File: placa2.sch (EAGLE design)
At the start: 9 parts

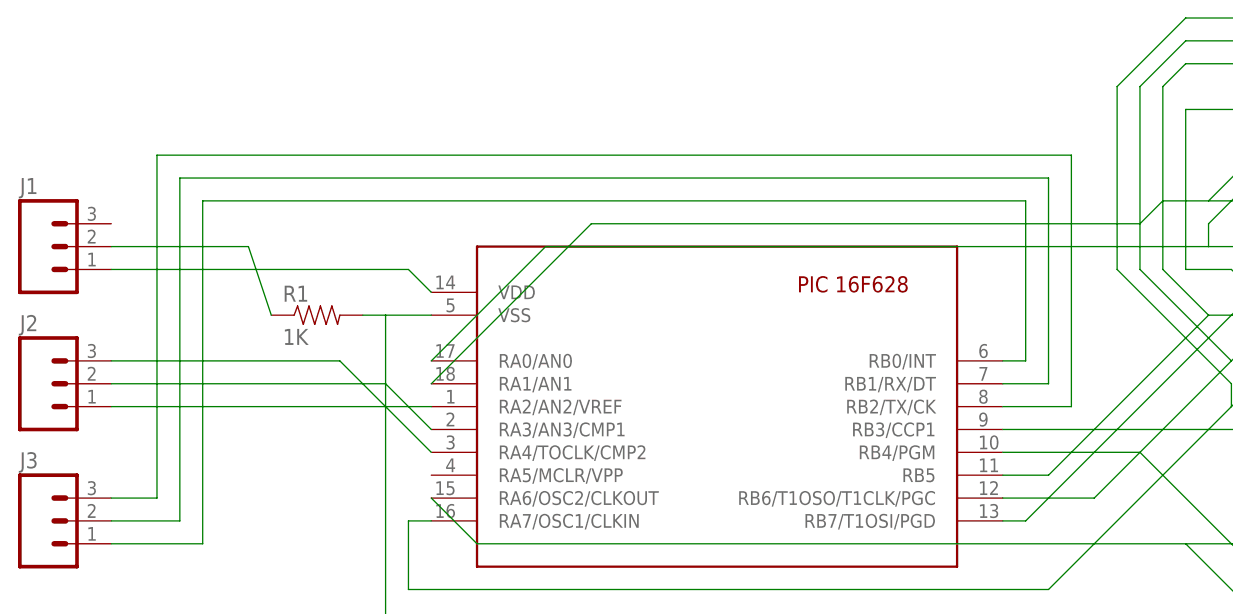
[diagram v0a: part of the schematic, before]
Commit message: feito
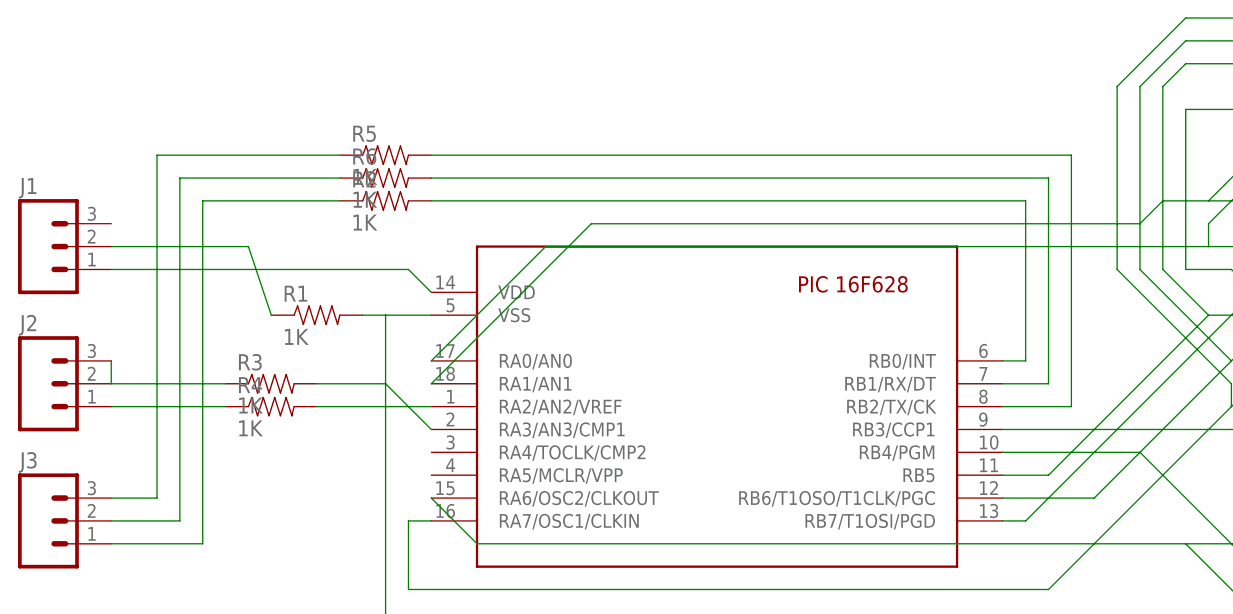
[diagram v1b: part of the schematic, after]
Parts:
- added R2, R3, R4, R5, R6: 1K, SparkFun-Resistors:1KOHM-1/4W-1%(PTH)
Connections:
- new net N$14: J3.2, R6.1
- new net N$16: J3.1, R2.1
- new net N$21: R3.2, U$1.RA3/AN3/CMP1
- new net N$24: R4.2, U$1.RA2/AN2/VREF
- net N$3: now also R4.1; no longer U$1.RA2/AN2/VREF
- net N$5: now also J2.3, R3.1; no longer J2.2, U$1.RA3/AN3/CMP1
- net N$6: now also J3.3, R5.1; no longer J2.3, U$1.RA4/TOCLK/CMP2
- net N$7: now also R2.2; no longer J3.1
- net N$8: now also R6.2; no longer J3.2
- net N$9: now also R5.2; no longer J3.3
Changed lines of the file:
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@@
 <classes>
 <class number="0" name="default" width="0.8" drill="0">
-<clearance class="0" value="0.3"/>
+<clearance class="0" value="0.4"/>
 </class>
 </classes>
@@
 <part name="T1" library="transistor" deviceset="*-PNP-" device="TO92-EBC" technology="BC558B"/>
 <part name="T2" library="transistor" deviceset="*-PNP-" device="TO92-EBC" technology="BC558B"/>
+<part name="R3" library="SparkFun-Resistors" deviceset="1KOHM-1/4W-1%(PTH)" device="" value="1K"/>
+<part name="R4" library="SparkFun-Resistors" deviceset="1KOHM-1/4W-1%(PTH)" device="" value="1K"/>
+<part name="R5" library="SparkFun-Resistors" deviceset="1KOHM-1/4W-1%(PTH)" device="" value="1K"/>
+<part name="R6" library="SparkFun-Resistors" deviceset="1KOHM-1/4W-1%(PTH)" device="" value="1K"/>
+<part name="R2" library="SparkFun-Resistors" deviceset="1KOHM-1/4W-1%(PTH)" device="" value="1K"/>
 </parts>
 <sheets>
@@
 <instance part="T1" gate="G$1" x="109.22" y="-7.62" rot="R90"/>
 <instance part="T2" gate="G$1" x="172.72" y="-20.32" rot="R90"/>
+<instance part="R3" gate="G$1" x="-35.56" y="22.86"/>
+<instance part="R4" gate="G$1" x="-35.56" y="20.32"/>
+<instance part="R5" gate="G$1" x="-22.86" y="48.26"/>
+<instance part="R6" gate="G$1" x="-22.86" y="45.72"/>
+<instance part="R2" gate="G$1" x="-22.86" y="43.18"/>
 </instances>
 <busses>
@@
 <segment>
 <pinref part="J2" gate="J$1" pin="1"/>
-<pinref part="U$1" gate="G$1" pin="RA2/AN2/VREF"/>
-<wire x1="-53.34" y1="20.32" x2="-17.78" y2="20.32" width="0.1524" layer="91"/>
-</segment>
-</net>
-<net name="N$5" class="0">
-<segment>
-<pinref part="J2" gate="J$1" pin="2"/>
-<pinref part="U$1" gate="G$1" pin="RA3/AN3/CMP1"/>
-<wire x1="-53.34" y1="22.86" x2="-22.86" y2="22.86" width="0.1524" layer="91"/>
-<wire x1="-22.86" y1="22.86" x2="-17.78" y2="17.78" width="0.1524" layer="91"/>
-</segment>
-</net>
-<net name="N$6" class="0">
-<segment>
-<pinref part="J2" gate="J$1" pin="3"/>
-<pinref part="U$1" gate="G$1" pin="RA4/TOCLK/CMP2"/>
-<wire x1="-53.34" y1="25.4" x2="-27.94" y2="25.4" width="0.1524" layer="91"/>
-<wire x1="-27.94" y1="25.4" x2="-17.78" y2="15.24" width="0.1524" layer="91"/>
+<wire x1="-53.34" y1="20.32" x2="-40.64" y2="20.32" width="0.1524" layer="91"/>
+<pinref part="R4" gate="G$1" pin="1"/>
 </segment>
 </net>
@@
 <net name="N$7" class="0">
 <segment>
-<pinref part="J3" gate="J$1" pin="1"/>
-<wire x1="-53.34" y1="5.08" x2="-43.18" y2="5.08" width="0.1524" layer="91"/>
-<wire x1="-43.18" y1="5.08" x2="-43.18" y2="43.18" width="0.1524" layer="91"/>
-<wire x1="-43.18" y1="43.18" x2="48.26" y2="43.18" width="0.1524" layer="91"/>
+<wire x1="-17.78" y1="43.18" x2="48.26" y2="43.18" width="0.1524" layer="91"/>
 <wire x1="48.26" y1="43.18" x2="48.26" y2="25.4" width="0.1524" layer="91"/>
 <pinref part="U$1" gate="G$1" pin="RB0/INT"/>
 <wire x1="48.26" y1="25.4" x2="45.72" y2="25.4" width="0.1524" layer="91"/>
+<pinref part="R2" gate="G$1" pin="2"/>
 </segment>
 </net>
 <net name="N$8" class="0">
 <segment>
-<pinref part="J3" gate="J$1" pin="2"/>
-<wire x1="-53.34" y1="7.62" x2="-45.72" y2="7.62" width="0.1524" layer="91"/>
-<wire x1="-45.72" y1="7.62" x2="-45.72" y2="45.72" width="0.1524" layer="91"/>
-<wire x1="-45.72" y1="45.72" x2="50.8" y2="45.72" width="0.1524" layer="91"/>
+<wire x1="-17.78" y1="45.72" x2="50.8" y2="45.72" width="0.1524" layer="91"/>
 <wire x1="50.8" y1="45.72" x2="50.8" y2="22.86" width="0.1524" layer="91"/>
 <pinref part="U$1" gate="G$1" pin="RB1/RX/DT"/>
 <wire x1="50.8" y1="22.86" x2="45.72" y2="22.86" width="0.1524" layer="91"/>
+<pinref part="R6" gate="G$1" pin="2"/>
 </segment>
 </net>
 <net name="N$9" class="0">
 <segment>
-<pinref part="J3" gate="J$1" pin="3"/>
-<wire x1="-53.34" y1="10.16" x2="-48.26" y2="10.16" width="0.1524" layer="91"/>
-<wire x1="-48.26" y1="10.16" x2="-48.26" y2="48.26" width="0.1524" layer="91"/>
-<wire x1="-48.26" y1="48.26" x2="53.34" y2="48.26" width="0.1524" layer="91"/>
+<wire x1="-17.78" y1="48.26" x2="53.34" y2="48.26" width="0.1524" layer="91"/>
 <wire x1="53.34" y1="48.26" x2="53.34" y2="20.32" width="0.1524" layer="91"/>
 <pinref part="U$1" gate="G$1" pin="RB2/TX/CK"/>
 <wire x1="53.34" y1="20.32" x2="45.72" y2="20.32" width="0.1524" layer="91"/>
+<pinref part="R5" gate="G$1" pin="2"/>
 </segment>
 </net>
@@
 </segment>
 </net>
+<net name="N$6" class="0">
+<segment>
+<pinref part="R5" gate="G$1" pin="1"/>
+<pinref part="J3" gate="J$1" pin="3"/>
+<wire x1="-53.34" y1="10.16" x2="-48.26" y2="10.16" width="0.1524" layer="91"/>
+<wire x1="-48.26" y1="10.16" x2="-48.26" y2="48.26" width="0.1524" layer="91"/>
+<wire x1="-48.26" y1="48.26" x2="-27.94" y2="48.26" width="0.1524" layer="91"/>
+</segment>
+</net>
+<net name="N$14" class="0">
+<segment>
+<pinref part="R6" gate="G$1" pin="1"/>
+<pinref part="J3" gate="J$1" pin="2"/>
+<wire x1="-53.34" y1="7.62" x2="-45.72" y2="7.62" width="0.1524" layer="91"/>
+<wire x1="-45.72" y1="7.62" x2="-45.72" y2="45.72" width="0.1524" layer="91"/>
+<wire x1="-45.72" y1="45.72" x2="-27.94" y2="45.72" width="0.1524" layer="91"/>
+</segment>
+</net>
+<net name="N$16" class="0">
+<segment>
+<pinref part="R2" gate="G$1" pin="1"/>
+<pinref part="J3" gate="J$1" pin="1"/>
+<wire x1="-53.34" y1="5.08" x2="-43.18" y2="5.08" width="0.1524" layer="91"/>
+<wire x1="-43.18" y1="5.08" x2="-43.18" y2="43.18" width="0.1524" layer="91"/>
+<wire x1="-43.18" y1="43.18" x2="-27.94" y2="43.18" width="0.1524" layer="91"/>
+</segment>
+</net>
+<net name="N$21" class="0">
+<segment>
+<pinref part="U$1" gate="G$1" pin="RA3/AN3/CMP1"/>
+<pinref part="R3" gate="G$1" pin="2"/>
+<wire x1="-30.48" y1="22.86" x2="-22.86" y2="22.86" width="0.1524" layer="91"/>
+<wire x1="-22.86" y1="22.86" x2="-17.78" y2="17.78" width="0.1524" layer="91"/>
+</segment>
+</net>
+<net name="N$24" class="0">
+<segment>
+<pinref part="U$1" gate="G$1" pin="RA2/AN2/VREF"/>
+<pinref part="R4" gate="G$1" pin="2"/>
+<wire x1="-30.48" y1="20.32" x2="-17.78" y2="20.32" width="0.1524" layer="91"/>
+</segment>
+</net>
+<net name="N$5" class="0">
+<segment>
+<pinref part="R3" gate="G$1" pin="1"/>
+<pinref part="J2" gate="J$1" pin="3"/>
+<wire x1="-40.64" y1="22.86" x2="-53.34" y2="22.86" width="0.1524" layer="91"/>
+<wire x1="-53.34" y1="22.86" x2="-53.34" y2="25.4" width="0.1524" layer="91"/>
+</segment>
+</net>
